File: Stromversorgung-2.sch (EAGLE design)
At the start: 16 parts, among them J1 DCJ0202, U1 TSR 2-2450, U2 TSR 1-2433, U3 TSR 2-2450, X1 Ein/Aus, X2 MAC64L

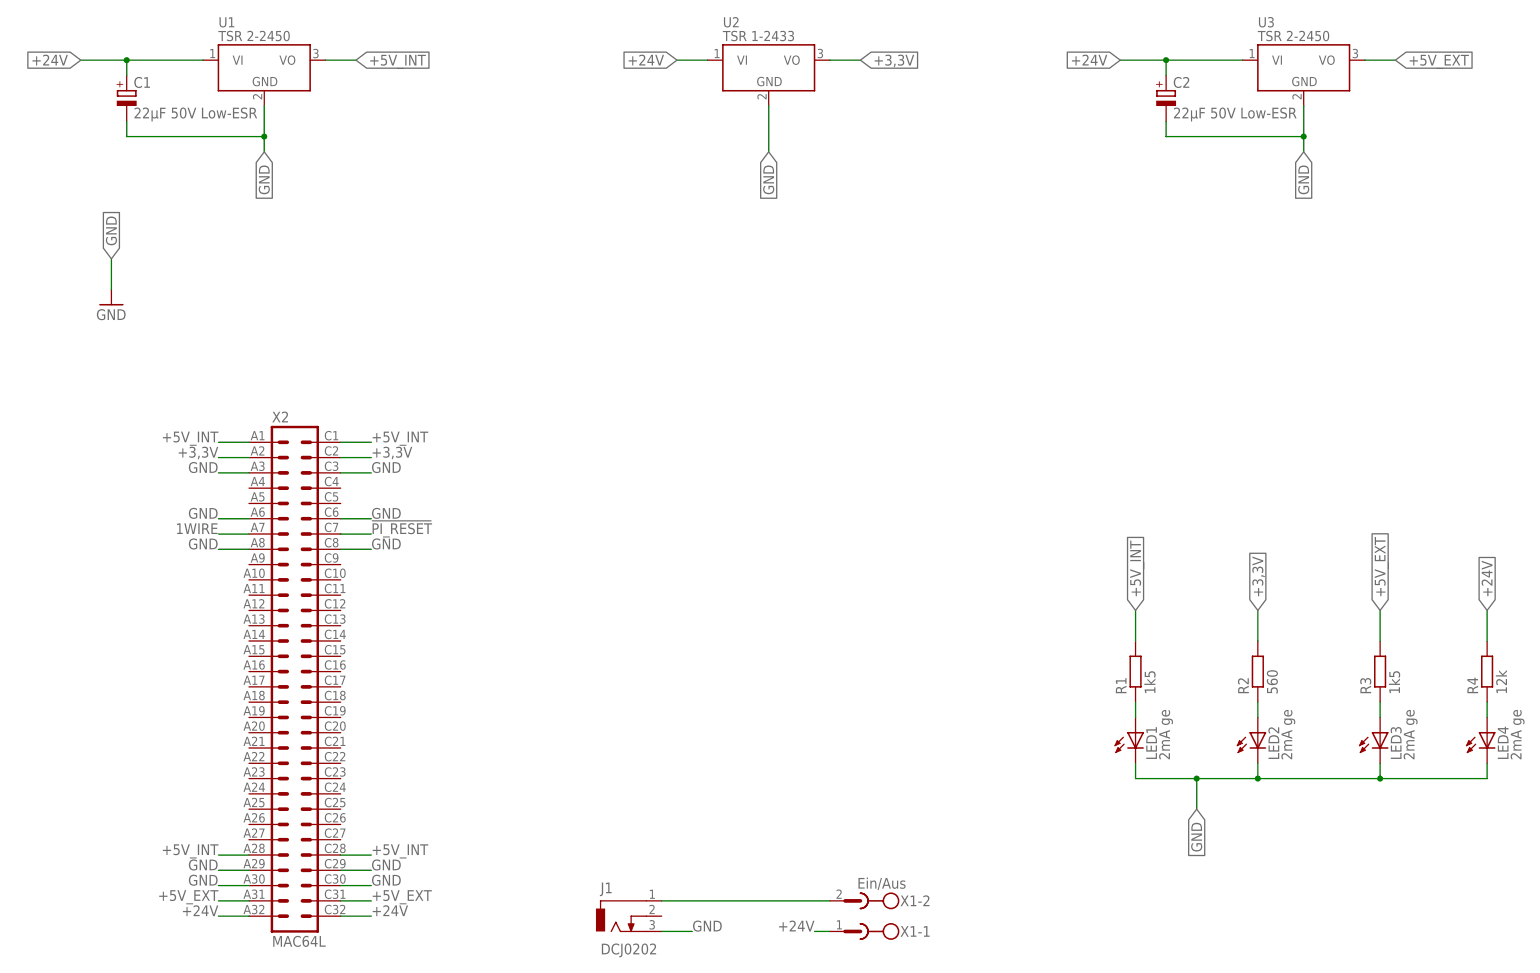
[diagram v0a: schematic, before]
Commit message: Layouts angepasst
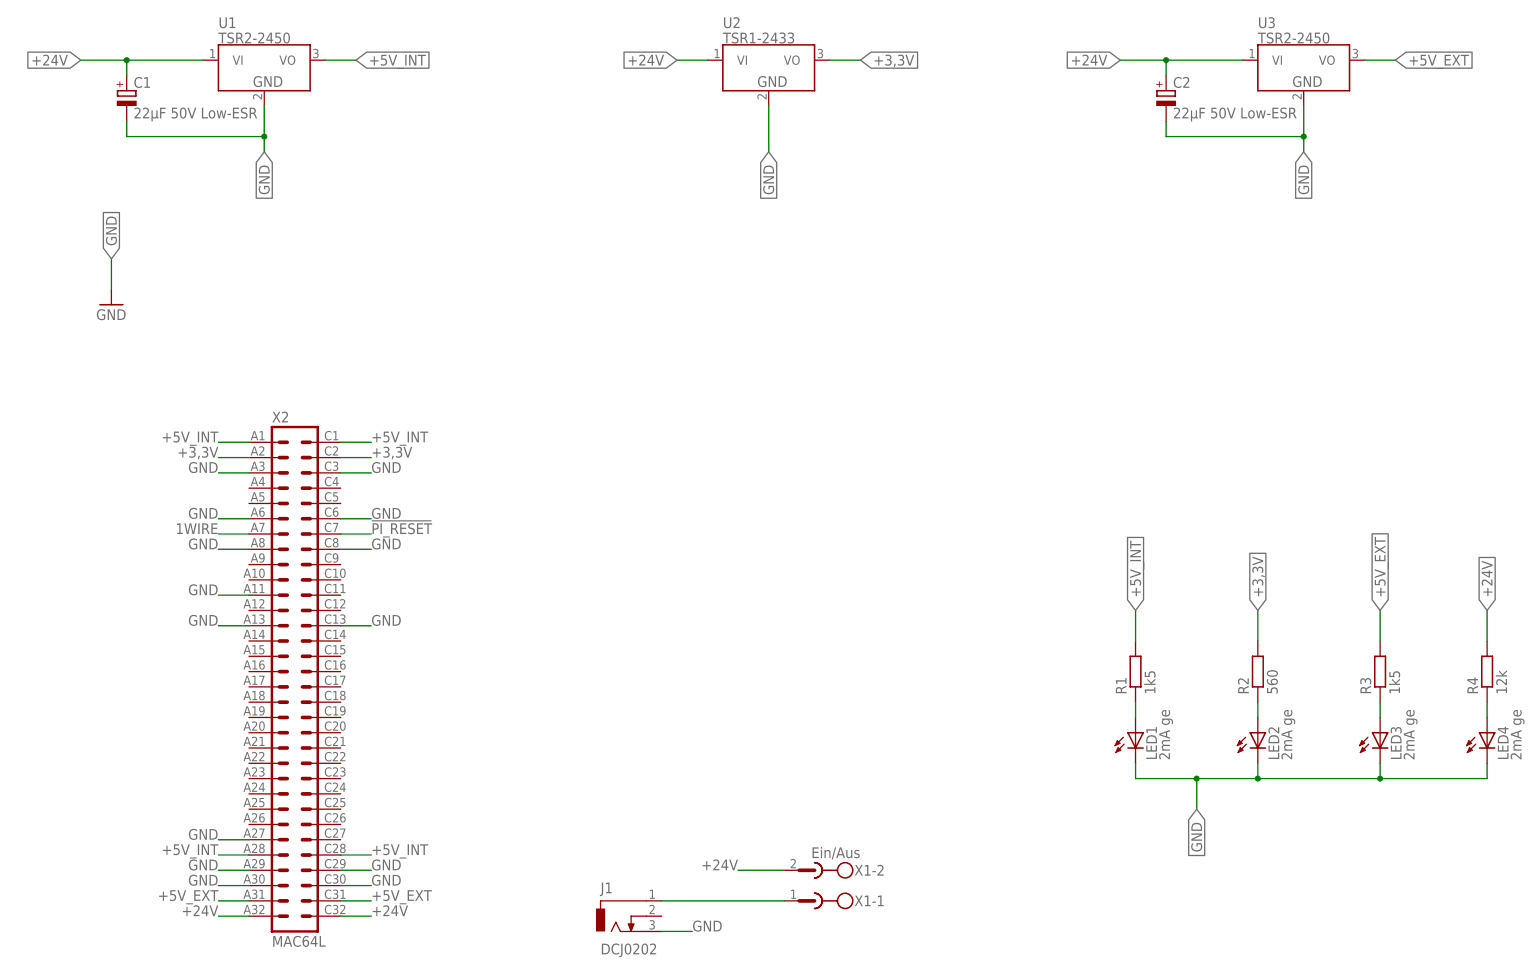
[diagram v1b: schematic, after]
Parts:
- R1, R2, R3, R4: device rcl:R-EU_0204/5 -> rcl:R-EU_R1206
- U1, U3: value TSR 2-2450 -> TSR2-2450; device _traco_tsr-1:TSR_1-2450 -> TSR:TSR2-2450
- U2: value TSR 1-2433 -> TSR1-2433; device _traco_tsr-1:TSR_1-2433 -> TSR:TSR1-2433
- X1: device con-phoenix-508:MSTBV2 -> con-phoenix-508:MSTBA2
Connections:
- net +24V: now also X1-2.1; no longer X1-1.1
- net GND: now also X2.A11, X2.A13, X2.A27, X2.C13
- net N$1: now also X1-1.1; no longer X1-2.1
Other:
- moved on the sheet: X1-1, X1-2
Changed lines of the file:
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@@
 <class number="0" name="default" width="0" drill="0">
 </class>
-<class number="1" name="24V" width="0.8128" drill="0">
+<class number="1" name="24V" width="0" drill="0">
 <clearance class="1" value="0.4064"/>
 </class>
 </classes>
 <parts>
-<part name="X1" library="con-phoenix-508" deviceset="MSTBV2" device="" value="Ein/Aus"/>
+<part name="X1" library="con-phoenix-508" deviceset="MSTBA2" device="" value="Ein/Aus"/>
 <part name="LED1" library="led" deviceset="LED" device="3MM" value="2mA ge"/>
 <part name="LED2" library="led" deviceset="LED" device="3MM" value="2mA ge"/>
 <part name="LED3" library="led" deviceset="LED" device="3MM" value="2mA ge"/>
-<part name="R1" library="rcl" deviceset="R-EU_" device="0204/5" value="1k5"/>
-<part name="R2" library="rcl" deviceset="R-EU_" device="0204/5" value="560"/>
-<part name="R3" library="rcl" deviceset="R-EU_" device="0204/5" value="1k5"/>
-<part name="U1" library="_traco_tsr-1" deviceset="TSR_1-*" device="" technology="2450" value="TSR 2-2450"/>
-<part name="U2" library="_traco_tsr-1" deviceset="TSR_1-*" device="" technology="2433" value="TSR 1-2433"/>
-<part name="U3" library="_traco_tsr-1" deviceset="TSR_1-*" device="" technology="2450" value="TSR 2-2450"/>
+<part name="R1" library="rcl" deviceset="R-EU_" device="R1206" value="1k5"/>
+<part name="R2" library="rcl" deviceset="R-EU_" device="R1206" value="560"/>
+<part name="R3" library="rcl" deviceset="R-EU_" device="R1206" value="1k5"/>
+<part name="U1" library="TSR" deviceset="TSR2-*" device="" technology="2450" value="TSR2-2450"/>
+<part name="U2" library="TSR" deviceset="TSR1-*" device="" technology="2433" value="TSR1-2433"/>
+<part name="U3" library="TSR" deviceset="TSR2-*" device="" technology="2450" value="TSR2-2450"/>
 <part name="FRAME1" library="frames" deviceset="A4L-LOC" device=""/>
 <part name="GND1" library="supply1" deviceset="GND" device=""/>
@@
 <part name="C1" library="rcl" deviceset="CPOL-EU" device="E2-5" value="22µF 50V Low-ESR"/>
 <part name="C2" library="rcl" deviceset="CPOL-EU" device="E2-5" value="22µF 50V Low-ESR"/>
-<part name="R4" library="rcl" deviceset="R-EU_" device="0204/5" value="12k"/>
+<part name="R4" library="rcl" deviceset="R-EU_" device="R1206" value="12k"/>
 <part name="LED4" library="led" deviceset="LED" device="3MM" value="2mA ge"/>
 </parts>
@@
 </plain>
 <instances>
-<instance part="X1" gate="-1" x="139.7" y="7.62" rot="R180"/>
-<instance part="X1" gate="-2" x="139.7" y="12.7" rot="R180"/>
+<instance part="X1" gate="-1" x="132.08" y="12.7" rot="R180"/>
+<instance part="X1" gate="-2" x="132.08" y="17.78" rot="R180"/>
 <instance part="LED1" gate="G$1" x="185.42" y="40.64"/>
 <instance part="LED2" gate="G$1" x="205.74" y="40.64"/>
@@
 <instance part="R2" gate="G$1" x="205.74" y="50.8" rot="R90"/>
 <instance part="R3" gate="G$1" x="226.06" y="50.8" rot="R90"/>
-<instance part="U1" gate="G$1" x="40.64" y="152.4"/>
-<instance part="U2" gate="G$1" x="124.46" y="152.4"/>
-<instance part="U3" gate="G$1" x="213.36" y="152.4"/>
+<instance part="U1" gate="U1" x="40.64" y="152.4"/>
+<instance part="U2" gate="U1" x="124.46" y="152.4"/>
+<instance part="U3" gate="U1" x="213.36" y="152.4"/>
 <instance part="FRAME1" gate="G$1" x="-5.08" y="-5.08"/>
 <instance part="GND1" gate="1" x="15.24" y="111.76"/>
@@
 </segment>
 <segment>
-<pinref part="U1" gate="G$1" pin="VO"/>
+<pinref part="U1" gate="U1" pin="VO"/>
 <wire x1="50.8" y1="152.4" x2="55.88" y2="152.4" width="0.1524" layer="91"/>
 <label x="55.88" y="152.4" size="1.778" layer="95" xref="yes"/>
@@
 </segment>
 <segment>
-<pinref part="U3" gate="G$1" pin="VO"/>
+<pinref part="U3" gate="U1" pin="VO"/>
 <wire x1="223.52" y1="152.4" x2="228.6" y2="152.4" width="0.1524" layer="91"/>
 <label x="228.6" y="152.4" size="1.778" layer="95" xref="yes"/>
@@
 <segment>
 <label x="139.7" y="152.4" size="1.778" layer="95" xref="yes"/>
-<pinref part="U2" gate="G$1" pin="VO"/>
+<pinref part="U2" gate="U1" pin="VO"/>
 <wire x1="134.62" y1="152.4" x2="139.7" y2="152.4" width="0.1524" layer="91"/>
 </segment>
@@
 <net name="+24V" class="1">
 <segment>
-<pinref part="U1" gate="G$1" pin="VI"/>
+<pinref part="U1" gate="U1" pin="VI"/>
 <wire x1="30.48" y1="152.4" x2="17.78" y2="152.4" width="0.1524" layer="91"/>
 <label x="10.16" y="152.4" size="1.778" layer="95" rot="R180" xref="yes"/>
@@
 </segment>
 <segment>
-<pinref part="U3" gate="G$1" pin="VI"/>
+<pinref part="U3" gate="U1" pin="VI"/>
 <wire x1="203.2" y1="152.4" x2="190.5" y2="152.4" width="0.1524" layer="91"/>
 <label x="182.88" y="152.4" size="1.778" layer="95" rot="R180" xref="yes"/>
@@
 </segment>
 <segment>
-<pinref part="X1" gate="-1" pin="1"/>
-<wire x1="134.62" y1="7.62" x2="132.08" y2="7.62" width="0.1524" layer="91"/>
-<label x="132.08" y="7.62" size="1.778" layer="95" rot="MR0"/>
-</segment>
-<segment>
 <pinref part="R4" gate="G$1" pin="2"/>
 <wire x1="243.84" y1="55.88" x2="243.84" y2="60.96" width="0.1524" layer="91"/>
@@
 </segment>
 <segment>
-<pinref part="U2" gate="G$1" pin="VI"/>
+<pinref part="U2" gate="U1" pin="VI"/>
 <wire x1="109.22" y1="152.4" x2="114.3" y2="152.4" width="0.1524" layer="91"/>
 <label x="109.22" y="152.4" size="1.778" layer="95" rot="R180" xref="yes"/>
+</segment>
+<segment>
+<pinref part="X1" gate="-2" pin="1"/>
+<wire x1="127" y1="17.78" x2="119.38" y2="17.78" width="0.1524" layer="91"/>
+<label x="119.38" y="17.78" size="1.778" layer="95" rot="MR0"/>
 </segment>
 </net>
@@
 </segment>
 <segment>
-<pinref part="U1" gate="G$1" pin="GND"/>
+<pinref part="U1" gate="U1" pin="GND"/>
 <wire x1="40.64" y1="144.78" x2="40.64" y2="139.7" width="0.1524" layer="91"/>
 <label x="40.64" y="137.16" size="1.778" layer="95" rot="R270" xref="yes"/>
@@
 </segment>
 <segment>
-<pinref part="U2" gate="G$1" pin="GND"/>
+<pinref part="U2" gate="U1" pin="GND"/>
 <wire x1="124.46" y1="144.78" x2="124.46" y2="137.16" width="0.1524" layer="91"/>
 <label x="124.46" y="137.16" size="1.778" layer="95" rot="R270" xref="yes"/>
 </segment>
 <segment>
-<pinref part="U3" gate="G$1" pin="GND"/>
+<pinref part="U3" gate="U1" pin="GND"/>
 <wire x1="213.36" y1="144.78" x2="213.36" y2="139.7" width="0.1524" layer="91"/>
 <label x="213.36" y="137.16" size="1.778" layer="95" rot="R270" xref="yes"/>
@@
 <label x="58.42" y="15.24" size="1.778" layer="95"/>
 </segment>
-</net>
-<net name="N$1" class="1">
-<segment>
-<pinref part="J1" gate="G$1" pin="1"/>
-<pinref part="X1" gate="-2" pin="1"/>
-<wire x1="106.68" y1="12.7" x2="134.62" y2="12.7" width="0.1524" layer="91"/>
+<segment>
+<pinref part="X2" gate="G$1" pin="A11"/>
+<wire x1="38.1" y1="63.5" x2="33.02" y2="63.5" width="0.1524" layer="91"/>
+<label x="33.02" y="63.5" size="1.778" layer="95" rot="MR0"/>
+</segment>
+<segment>
+<pinref part="X2" gate="G$1" pin="A13"/>
+<wire x1="38.1" y1="58.42" x2="33.02" y2="58.42" width="0.1524" layer="91"/>
+<label x="33.02" y="58.42" size="1.778" layer="95" rot="MR0"/>
+</segment>
+<segment>
+<pinref part="X2" gate="G$1" pin="C13"/>
+<wire x1="53.34" y1="58.42" x2="58.42" y2="58.42" width="0.1524" layer="91"/>
+<label x="58.42" y="58.42" size="1.778" layer="95"/>
+</segment>
+<segment>
+<pinref part="X2" gate="G$1" pin="A27"/>
+<wire x1="38.1" y1="22.86" x2="33.02" y2="22.86" width="0.1524" layer="91"/>
+<label x="33.02" y="22.86" size="1.778" layer="95" rot="MR0"/>
 </segment>
 </net>
@@
 </segment>
 </net>
+<net name="N$1" class="0">
+<segment>
+<pinref part="J1" gate="G$1" pin="1"/>
+<pinref part="X1" gate="-1" pin="1"/>
+<wire x1="106.68" y1="12.7" x2="127" y2="12.7" width="0.1524" layer="91"/>
+</segment>
+</net>
